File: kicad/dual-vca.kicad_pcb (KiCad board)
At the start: 2 copper layers, 0 parts

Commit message: Adding beginnings of panel files and routed more of the pcb
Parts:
- added C1: 560pF, Rumblesan_Standard_Parts:C_Rect_L7.0mm_W2.5mm_P5.00mm, F.Cu at (123.5, 58.5)
- added C10: 10uF, Rumblesan_Standard_Parts:CP_Radial_D5.0mm_P2.00mm, F.Cu at (135.7, 37.8)
- added C11: 100nF, Rumblesan_Standard_Parts:C_Rect_L7.0mm_W2.5mm_P5.00mm, F.Cu at (123.0, 106.9)
- added C12: 100nF, Rumblesan_Standard_Parts:C_Rect_L7.0mm_W2.5mm_P5.00mm, F.Cu at (125.0, 66.2)
- added C13: 100nF, Rumblesan_Standard_Parts:C_Rect_L7.0mm_W2.5mm_P5.00mm, F.Cu at (138.0, 124.7)
- added C14: 100nF, Rumblesan_Standard_Parts:C_Rect_L7.0mm_W2.5mm_P5.00mm, F.Cu at (118.1, 125.1)
- added C15: 470nF, Rumblesan_Standard_Parts:C_Rect_L7.0mm_W2.5mm_P5.00mm, F.Cu at (130.6, 48.8)
- added C16: 470nF, Rumblesan_Standard_Parts:C_Rect_L7.0mm_W2.5mm_P5.00mm, F.Cu at (137.7, 61.5)
- added C2: 560pF, Rumblesan_Standard_Parts:C_Rect_L7.0mm_W2.5mm_P5.00mm, F.Cu at (113.5, 134.5)
- added C3: 100pF, Rumblesan_Standard_Parts:C_Rect_L7.0mm_W2.5mm_P5.00mm, F.Cu at (133.0, 129.5)
- added C4: 100pF, Rumblesan_Standard_Parts:C_Rect_L7.0mm_W2.5mm_P5.00mm, F.Cu at (118.1, 127.8)
- added C5: 560pF, Rumblesan_Standard_Parts:C_Rect_L7.0mm_W2.5mm_P5.00mm, F.Cu at (133.2, 109.1)
- added C6: 560pF, Rumblesan_Standard_Parts:C_Rect_L7.0mm_W2.5mm_P5.00mm, F.Cu at (116.1, 61.4)
- added C7: 100pF, Rumblesan_Standard_Parts:C_Rect_L7.0mm_W2.5mm_P5.00mm, F.Cu at (133.5, 120.5)
- added C8: 100pF, Rumblesan_Standard_Parts:C_Rect_L7.0mm_W2.5mm_P5.00mm, F.Cu at (118.1, 117.5)
- added C9: 10uF, Rumblesan_Standard_Parts:CP_Radial_D5.0mm_P2.00mm, F.Cu at (130.8, 38.0)
- added D1: 1N5818, Rumblesan_Standard_Parts:D_DO-41_SOD81_P10.16mm_Horizontal, F.Cu at (124.7, 35.6)
- added D2: 1N5818, Rumblesan_Standard_Parts:D_DO-41_SOD81_P10.16mm_Horizontal, F.Cu at (124.5, 32.0)
- added H1: MountingHole_Pad, MountingHole:MountingHole_3.2mm_M3_DIN965_Pad, F.Cu at (94.5, 134.5)
- added H2: MountingHole_Pad, MountingHole:MountingHole_3.2mm_M3_DIN965_Pad, F.Cu at (94.5, 51.5)
- added H3: MountingHole_Pad, MountingHole:MountingHole_3.2mm_M3_DIN965_Pad, F.Cu at (125.5, 51.5)
- added H4: MountingHole_Pad, MountingHole:MountingHole_3.2mm_M3_DIN965_Pad, F.Cu at (125.5, 134.5)
- added J1: Eurorack Mono Jack, Rumblesan_Standard_Parts:Jack_3.5mm_QingPu_WQP-PJ398SM_Vertical, B.Cu at (102.0, 97.5)
- added J11: Conn_01x06_Socket, Connector_PinSocket_2.54mm:PinSocket_1x06_P2.54mm_Vertical, F.Cu at (107.0, 87.0)
- added J12: Conn_01x06_Pin, Connector_PinHeader_2.54mm:PinHeader_1x06_P2.54mm_Vertical, B.Cu at (117.9, 87.6)
- added J2: Eurorack Mono Jack, Rumblesan_Standard_Parts:Jack_3.5mm_QingPu_WQP-PJ398SM_Vertical, B.Cu at (87.0, 97.5)
- added J3: Eurorack Mono Jack, Rumblesan_Standard_Parts:Jack_3.5mm_QingPu_WQP-PJ398SM_Vertical, B.Cu at (102.0, 112.5)
- added J4: Eurorack Mono Jack, Rumblesan_Standard_Parts:Jack_3.5mm_QingPu_WQP-PJ398SM_Vertical, B.Cu at (87.0, 112.5)
- added J5: Eurorack Power Small, Eurorack_Power:Eurorack_PowerHeader_2x05_P2.54mm_Shrouded, F.Cu at (116.0, 38.5)
- added J6: Eurorack Mono Jack, Rumblesan_Standard_Parts:Jack_3.5mm_QingPu_WQP-PJ398SM_Vertical, B.Cu at (102.0, 127.5)
- added J7: Eurorack Mono Jack, Rumblesan_Standard_Parts:Jack_3.5mm_QingPu_WQP-PJ398SM_Vertical, B.Cu at (87.0, 127.5)
- added J8: Conn_01x06_Pin, Connector_PinHeader_2.54mm:PinHeader_1x06_P2.54mm_Vertical, B.Cu at (138.0, 87.0)
- added J9: Conn_01x06_Socket, Connector_PinSocket_2.54mm:PinSocket_1x06_P2.54mm_Vertical, F.Cu at (82.0, 87.0)
- added R1: 22k, Rumblesan_Standard_Parts:R_Axial_DIN0207_L6.3mm_D2.5mm_P10.16mm_Horizontal, F.Cu at (97.0, 85.7)
- added R10: 510r, Rumblesan_Standard_Parts:R_Axial_DIN0207_L6.3mm_D2.5mm_P10.16mm_Horizontal, F.Cu at (113.4, 99.2)
- added R11: 510r, Rumblesan_Standard_Parts:R_Axial_DIN0207_L6.3mm_D2.5mm_P10.16mm_Horizontal, F.Cu at (107.0, 32.0)
- added R12: 510r, Rumblesan_Standard_Parts:R_Axial_DIN0207_L6.3mm_D2.5mm_P10.16mm_Horizontal, F.Cu at (81.9, 32.0)
- added R13: 47k, Rumblesan_Standard_Parts:R_Axial_DIN0207_L6.3mm_D2.5mm_P10.16mm_Horizontal, F.Cu at (136.3, 101.3)
- added R14: 510r, Rumblesan_Standard_Parts:R_Axial_DIN0207_L6.3mm_D2.5mm_P10.16mm_Horizontal, F.Cu at (133.1, 91.2)
- added R15: 47k, Rumblesan_Standard_Parts:R_Axial_DIN0207_L6.3mm_D2.5mm_P10.16mm_Horizontal, F.Cu at (113.8, 66.5)
- added R16: 510r, Rumblesan_Standard_Parts:R_Axial_DIN0207_L6.3mm_D2.5mm_P10.16mm_Horizontal, F.Cu at (119.1, 66.3)
- added R17: 47k, Rumblesan_Standard_Parts:R_Axial_DIN0207_L6.3mm_D2.5mm_P10.16mm_Horizontal, F.Cu at (137.0, 121.0)
- added R18: 47k, Rumblesan_Standard_Parts:R_Axial_DIN0207_L6.3mm_D2.5mm_P10.16mm_Horizontal, F.Cu at (115.1, 127.0)
- added R19: 510r, Rumblesan_Standard_Parts:R_Axial_DIN0207_L6.3mm_D2.5mm_P10.16mm_Horizontal, F.Cu at (94.5, 117.5)
- added R2: 22k, Rumblesan_Standard_Parts:R_Axial_DIN0207_L6.3mm_D2.5mm_P10.16mm_Horizontal, F.Cu at (93.0, 86.7)
- added R20: 510r, Rumblesan_Standard_Parts:R_Axial_DIN0207_L6.3mm_D2.5mm_P10.16mm_Horizontal, F.Cu at (94.5, 103.8)
- added R21: 3k6, Rumblesan_Standard_Parts:R_Axial_DIN0207_L6.3mm_D2.5mm_P10.16mm_Horizontal, F.Cu at (133.9, 52.1)
- added R22: 24k, Rumblesan_Standard_Parts:R_Axial_DIN0207_L6.3mm_D2.5mm_P10.16mm_Horizontal, F.Cu at (137.9, 52.1)
- added R3: 20M, Rumblesan_Standard_Parts:R_Axial_DIN0207_L6.3mm_D2.5mm_P10.16mm_Horizontal, F.Cu at (134.6, 71.6)
- added R4: 47k, Rumblesan_Standard_Parts:R_Axial_DIN0207_L6.3mm_D2.5mm_P10.16mm_Horizontal, F.Cu at (131.6, 71.6)
- added R5: 100k, Rumblesan_Standard_Parts:R_Axial_DIN0207_L6.3mm_D2.5mm_P10.16mm_Horizontal, F.Cu at (101.5, 72.5)
- added R6: 510r, Rumblesan_Standard_Parts:R_Axial_DIN0207_L6.3mm_D2.5mm_P10.16mm_Horizontal, F.Cu at (128.5, 71.6)
- added R7: 20M, Rumblesan_Standard_Parts:R_Axial_DIN0207_L6.3mm_D2.5mm_P10.16mm_Horizontal, F.Cu at (119.8, 109.3)
- added R8: 47k, Rumblesan_Standard_Parts:R_Axial_DIN0207_L6.3mm_D2.5mm_P10.16mm_Horizontal, F.Cu at (116.6, 109.3)
- added R9: 100k, Rumblesan_Standard_Parts:R_Axial_DIN0207_L6.3mm_D2.5mm_P10.16mm_Horizontal, F.Cu at (88.0, 73.0)
- added RV1: 20kB, Rumblesan_Standard_Parts:Potentiometer_Alpha_RD901F-40-00D_Single_Vertical, B.Cu at (102.0, 59.5)
- added RV2: 20kB, Rumblesan_Standard_Parts:Potentiometer_Alpha_RD901F-40-00D_Single_Vertical, B.Cu at (87.0, 59.5)
- added RV3: 10kB, Rumblesan_Standard_Parts:Potentiometer_Alpha_RD901F-40-00D_Single_Vertical, B.Cu at (102.0, 39.5)
- added RV4: 10kB, Rumblesan_Standard_Parts:Potentiometer_Alpha_RD901F-40-00D_Single_Vertical, B.Cu at (87.0, 39.5)
- added U1: SSI2164, Package_DIP:DIP-16_W7.62mm_Socket, F.Cu at (129.5, 93.7)
- added U2: TL074, Package_DIP:DIP-14_W7.62mm_Socket, F.Cu at (121.7, 113.5)
- added U3: LM4040LP-10, Package_TO_SOT_THT:TO-92_Inline, F.Cu at (129.5, 45.2)
- added U4: LM4040LP-2.5, Package_TO_SOT_THT:TO-92_Inline, F.Cu at (137.9, 57.1)
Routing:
- net VCC: track 0.00 -> 106.3 mm
- net VEE: track 0.00 -> 105.4 mm
- net AREF_-2.5: track 0.00 -> 76.5 mm
- net /CV2_ATTN_MAIN: track 0.00 -> 67.9 mm
- net /RESPONSE2_TOP_MAIN: track 0.00 -> 63.9 mm
- net /RESPONSE1_TOP_MAIN: track 0.00 -> 54.6 mm
- net /CV1_ATTN_MAIN: track 0.00 -> 54.3 mm
- net AREF_+10: track 0.00 -> 50.2 mm
- net Net-(U2D--): track 0.00 -> 47.7 mm
- net Net-(U2A--): track 0.00 -> 47.0 mm
- net Net-(R10-Pad1): track 0.00 -> 46.5 mm
- net /RESPONSE2_TOP_CTRL: track 0.00 -> 36.7 mm
- net /RESPONSE2_WIPER_CTRL: track 0.00 -> 35.7 mm
- net /OUTPUT2_MAIN: track 0.00 -> 35.4 mm
- net /OUTPUT1_MAIN: track 0.00 -> 34.6 mm
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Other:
- board outline added: 60 x 108 mm

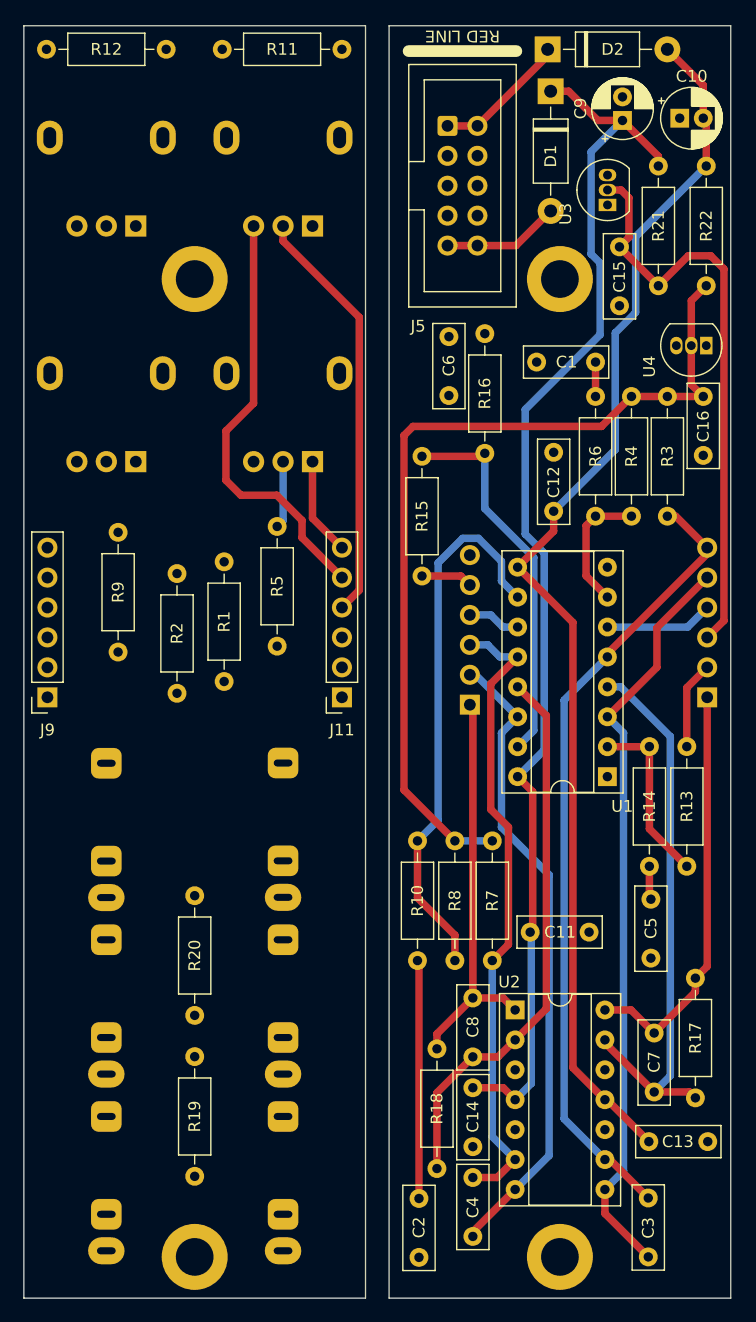
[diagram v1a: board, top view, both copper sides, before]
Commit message: Finishing routing PCBs
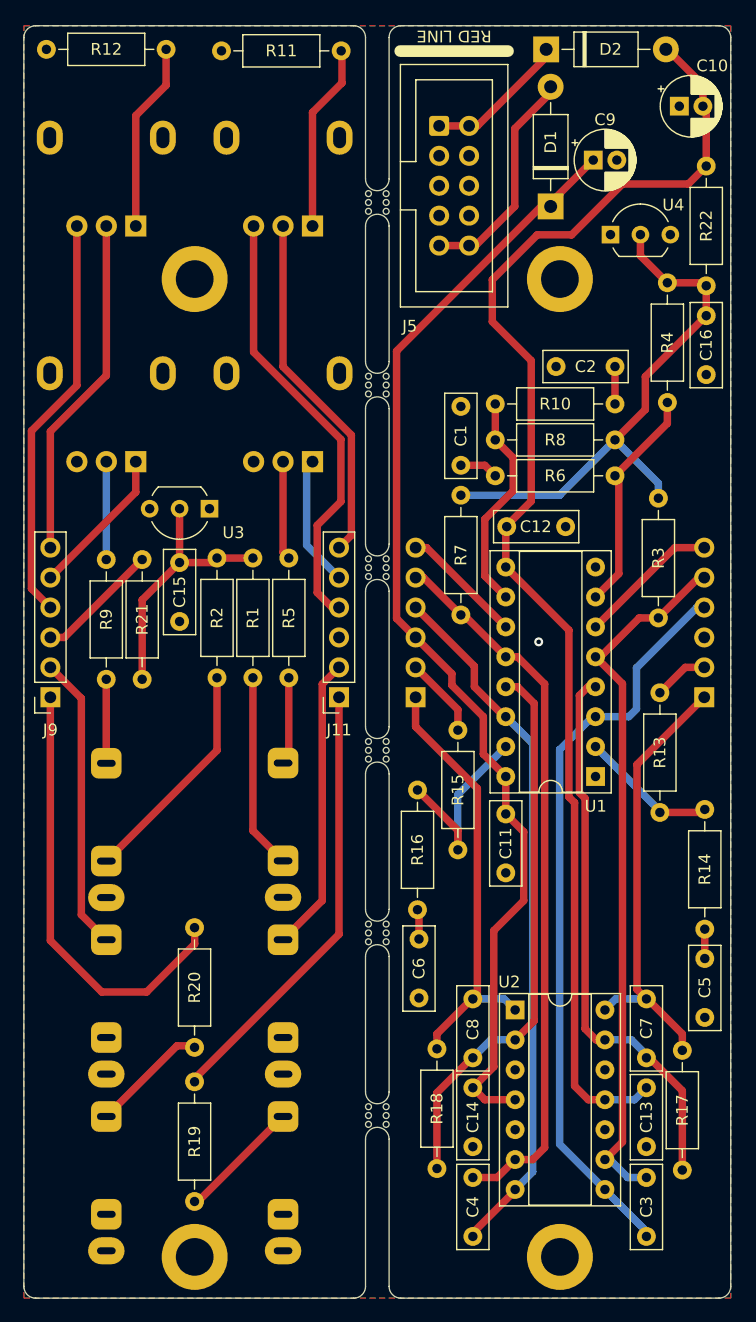
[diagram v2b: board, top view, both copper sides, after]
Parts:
- added mouse-bite-2mm-slot: VAL**, Panelization:mouse-bite-2mm-slot, F.Cu at (110.0, 45.0)
- added mouse-bite-2mm-slot: VAL**, Panelization:mouse-bite-2mm-slot, F.Cu at (110.0, 60.5)
- added mouse-bite-2mm-slot: VAL**, Panelization:mouse-bite-2mm-slot, F.Cu at (110.0, 76.0)
- added mouse-bite-2mm-slot: VAL**, Panelization:mouse-bite-2mm-slot, F.Cu at (110.0, 122.5)
- added mouse-bite-2mm-slot: VAL**, Panelization:mouse-bite-2mm-slot, F.Cu at (110.0, 91.5)
- added mouse-bite-2mm-slot: VAL**, Panelization:mouse-bite-2mm-slot, F.Cu at (110.0, 107.0)
- C1, C11, C12, C13, C14, C15, C16, C2, C3, C4, C5, C6, C7, C8: footprint Rumblesan_Standard_Parts:C_Rect_L7.0mm_W2.5mm_P5.00mm -> Capacitor_THT:C_Rect_L7.0mm_W2.5mm_P5.00mm
- C10, C9: footprint Rumblesan_Standard_Parts:CP_Radial_D5.0mm_P2.00mm -> Capacitor_THT:CP_Radial_D5.0mm_P2.00mm
- D1, D2: footprint Rumblesan_Standard_Parts:D_DO-41_SOD81_P10.16mm_Horizontal -> Diode_THT:D_DO-41_SOD81_P10.16mm_Horizontal
- R1, R10, R11, R12, R13, R14, R15, R16, R17, R18, R19, R2, R20, R21, R22, R3, R4, R5, R6, R7, R8, R9: footprint Rumblesan_Standard_Parts:R_Axial_DIN0207_L6.3mm_D2.5mm_P10.16mm_Horizontal -> Resistor_THT:R_Axial_DIN0207_L6.3mm_D2.5mm_P10.16mm_Horizontal
- U3, U4: footprint Package_TO_SOT_THT:TO-92_Inline -> Package_TO_SOT_THT:TO-92_Inline_Wide
- moved C2 76.5 mm to (125.2, 58.9), turned to 0 degrees
- moved C6 51.2 mm to (113.5, 112.5)
- moved R21 49.6 mm to (90.0, 75.3), turned to -90 degrees
- moved R8 46.2 mm to (130.2, 65.2), turned to 180 degrees
- moved C15 46.0 mm to (93.2, 75.6)
- moved U3 42.5 mm to (95.8, 71.0), turned to 180 degrees
- moved R10 40.7 mm to (130.2, 62.1), turned to 180 degrees
- moved R7 39.6 mm to (117.1, 69.8), turned to -90 degrees
- moved R16 39.2 mm to (113.4, 105.0)
- moved R15 23.4 mm to (116.8, 89.8)
- moved R4 20.0 mm to (134.6, 51.8), turned to -90 degrees
- moved R14 16.2 mm to (137.8, 106.7), turned to 90 degrees
- moved R13 14.9 mm to (134.0, 86.6), turned to -90 degrees
- moved R5 12.9 mm to (102.5, 85.3), turned to 90 degrees
- moved R20 12.9 mm to (94.5, 116.7), turned to 90 degrees
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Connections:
- C15 pad 1: AREF_+10 -> /10V_REF_CTRL
- J11 pad 3: /10V_REF_CTRL -> GND
- J11 pad 4: /RESPONSE2_WIPER_CTRL -> /RESPONSE2_TOP_CTRL
- J11 pad 5: /RESPONSE2_TOP_CTRL -> /CV2_ATTN_CTRL
- J11 pad 6: /CV2_ATTN_CTRL -> /RESPONSE2_WIPER_CTRL
- J12 pad 2: /RESPONSE1_TOP_MAIN -> /INPUT1_MAIN
- J12 pad 3: /CV1_ATTN_MAIN -> VCC
- J12 pad 4: /RESPONSE1_WIPER_MAIN -> /RESPONSE1_TOP_MAIN
- J12 pad 5: /INPUT1_MAIN -> /CV1_ATTN_MAIN
- J12 pad 6: GND -> /RESPONSE1_WIPER_MAIN
- J8 pad 3: AREF_+10 -> GND
- J8 pad 4: /RESPONSE2_WIPER_MAIN -> /RESPONSE2_TOP_MAIN
- J8 pad 5: /RESPONSE2_TOP_MAIN -> /CV2_ATTN_MAIN
- J8 pad 6: /CV2_ATTN_MAIN -> /RESPONSE2_WIPER_MAIN
- J9 pad 2: /RESPONSE1_TOP_CTRL -> /INPUT1_CTRL
- J9 pad 3: /CV1_ATTN_CTRL -> /VCC_CTRL
- J9 pad 4: /RESPONSE1_WIPER_CTRL -> /RESPONSE1_TOP_CTRL
- J9 pad 5: /INPUT1_CTRL -> /CV1_ATTN_CTRL
- J9 pad 6: GND -> /RESPONSE1_WIPER_CTRL
- R1 pad 1: Net-(J1-Tip_normalize) -> /10V_REF_CTRL
- R1 pad 2: /10V_REF_CTRL -> Net-(J1-Tip_normalize)
- R10 pad 1: Net-(R10-Pad1) -> Net-(C2-Pad2)
- R10 pad 2: Net-(C2-Pad2) -> Net-(R10-Pad2)
- R11 pad 1: Net-(R11-Pad1) -> GND
- R11 pad 2: GND -> Net-(R11-Pad2)
- R12 pad 1: Net-(R12-Pad1) -> GND
- R12 pad 2: GND -> Net-(R12-Pad2)
- R13 pad 1: Net-(R13-Pad1) -> /INPUT2_MAIN
- R13 pad 2: /INPUT2_MAIN -> Net-(R13-Pad2)
- R14 pad 1: Net-(R13-Pad1) -> Net-(C5-Pad2)
- R14 pad 2: Net-(C5-Pad2) -> Net-(R13-Pad2)
- R15 pad 1: Net-(R15-Pad1) -> /INPUT1_MAIN
- R15 pad 2: /INPUT1_MAIN -> Net-(R15-Pad2)
- R16 pad 1: Net-(R15-Pad1) -> Net-(C6-Pad2)
- R16 pad 2: Net-(C6-Pad2) -> Net-(R15-Pad2)
- R17 pad 1: Net-(U2D--) -> /OUTPUT2_MAIN
- R17 pad 2: /OUTPUT2_MAIN -> Net-(U2D--)
- R18 pad 1: Net-(U2A--) -> /OUTPUT1_MAIN
- R18 pad 2: /OUTPUT1_MAIN -> Net-(U2A--)
- R19 pad 1: /OUTPUT2_CTRL -> Net-(J6-Tip)
- R19 pad 2: Net-(J6-Tip) -> /OUTPUT2_CTRL
- R2 pad 1: Net-(J2-Tip_normalize) -> /10V_REF_CTRL
- R2 pad 2: /10V_REF_CTRL -> Net-(J2-Tip_normalize)
- R20 pad 1: /OUTPUT1_CTRL -> Net-(J7-Tip)
- R20 pad 2: Net-(J7-Tip) -> /OUTPUT1_CTRL
- R21 pad 1: AREF_+10 -> /VCC_CTRL
- R21 pad 2: VCC -> /10V_REF_CTRL
- R22 pad 1: AREF_-2.5 -> VEE
- R22 pad 2: VEE -> AREF_-2.5
- R3 pad 1: /CV2_ATTN_MAIN -> AREF_-2.5
- R3 pad 2: AREF_-2.5 -> /CV2_ATTN_MAIN
- R4 pad 1: Net-(R4-Pad1) -> AREF_-2.5
- R4 pad 2: AREF_-2.5 -> Net-(R4-Pad2)
- R5 pad 1: Net-(R5-Pad1) -> Net-(J1-Tip)
- R5 pad 2: Net-(J1-Tip) -> Net-(R5-Pad2)
- R6 pad 1: Net-(R4-Pad1) -> Net-(C1-Pad2)
- R6 pad 2: Net-(C1-Pad2) -> Net-(R4-Pad2)
- R7 pad 1: /CV1_ATTN_MAIN -> AREF_-2.5
- R7 pad 2: AREF_-2.5 -> /CV1_ATTN_MAIN
- R8 pad 1: Net-(R10-Pad1) -> AREF_-2.5
- R8 pad 2: AREF_-2.5 -> Net-(R10-Pad2)
- R9 pad 1: Net-(R9-Pad1) -> Net-(J2-Tip)
- R9 pad 2: Net-(J2-Tip) -> Net-(R9-Pad2)
- RV1 pad 2: Net-(R5-Pad1) -> Net-(R5-Pad2)
- RV2 pad 2: Net-(R9-Pad1) -> Net-(R9-Pad2)
- RV3 pad 1: Net-(R11-Pad1) -> Net-(R11-Pad2)
- RV4 pad 1: Net-(R12-Pad1) -> Net-(R12-Pad2)
- U1 pad 10: Net-(R10-Pad1) -> Net-(R10-Pad2)
- U1 pad 15: Net-(R15-Pad1) -> Net-(R15-Pad2)
- U1 pad 2: Net-(R13-Pad1) -> Net-(R13-Pad2)
- U1 pad 7: Net-(R4-Pad1) -> Net-(R4-Pad2)
- U3 pad 2: AREF_+10 -> /10V_REF_CTRL
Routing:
- net AREF_+10: track 50.2 -> 0.00 mm
- net Net-(R10-Pad1): track 46.5 -> 0.00 mm
- net /OUTPUT1_CTRL: track 0.00 -> 37.9 mm
- net /OUTPUT2_CTRL: track 0.00 -> 37.7 mm
- net /RESPONSE1_TOP_CTRL: track 0.00 -> 34.6 mm
- net Net-(R15-Pad1): track 32.6 -> 0.00 mm
- net AREF_-2.5: track 76.5 -> 46.1 mm
- net /RESPONSE1_WIPER_CTRL: track 0.00 -> 29.3 mm
- net /INPUT1_CTRL: track 0.00 -> 25.1 mm
- net /INPUT2_CTRL: track 0.00 -> 25.1 mm
- net /10V_REF_CTRL: track 0.00 -> 22.3 mm
- net Net-(J2-Tip_normalize): track 0.00 -> 19.4 mm
- net Net-(R4-Pad2): track 0.00 -> 19.3 mm
- net Net-(R10-Pad2): track 0.00 -> 18.8 mm
- net Net-(C2-Pad2): track 20.2 -> 3.18 mm
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- added copper zone on B.Cu, net GND
- added copper zone on F.Cu, net GND
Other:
- outline, holes or cut-outs redrawn
